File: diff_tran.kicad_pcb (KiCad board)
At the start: 2 copper layers, 28.7 x 13.8 mm, 30 parts, among them IC1 SN65LVDM176, IC2 SN65LVDM176, IC3 SN65LVDM176, IC4 SN65LVDM176, J1 SOLDER_JUMPER, J10 SOLDER_JUMPER, J11 SOLDER_JUMPER, J12 SOLDER_JUMPER, J2 SOLDER_JUMPER, J3 SOLDER_JUMPER, J4 SOLDER_JUMPER, J5 SOLDER_JUMPER, J6 SOLDER_JUMPER, J7 SOLDER_JUMPER, J8 SOLDER_JUMPER, J9 SOLDER_JUMPER, P1 CONN_02X03, P2 CONN_02X05

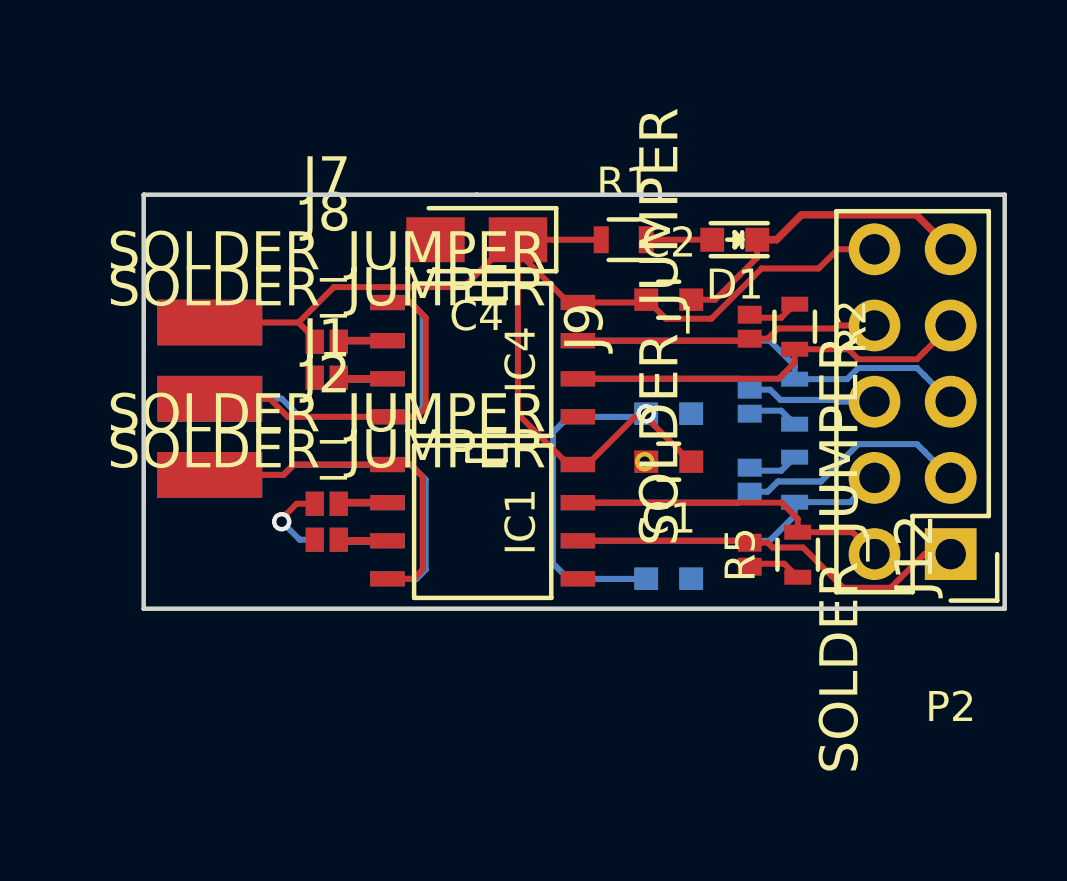
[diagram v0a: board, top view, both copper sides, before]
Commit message: Added some text, almost finished
Added some text, almost finished
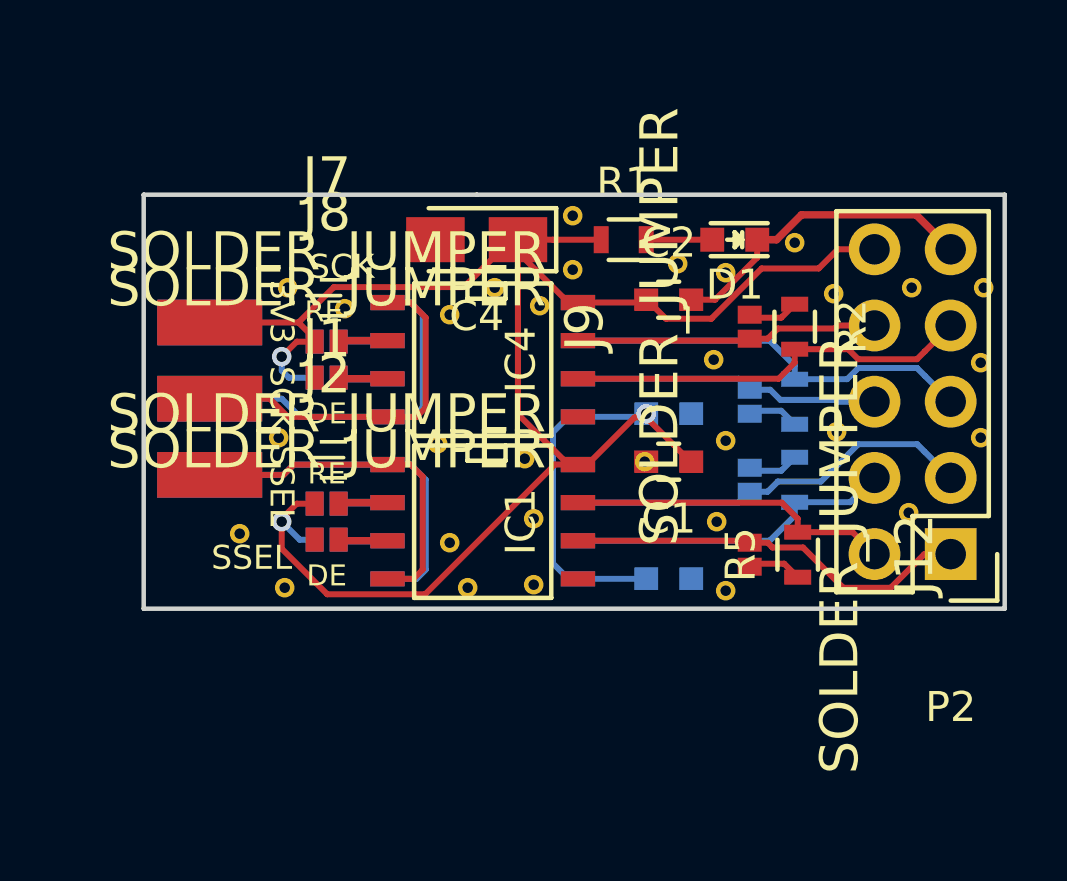
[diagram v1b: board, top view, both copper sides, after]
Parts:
- added ?: , LercheTech:Lerche_via_0.35_GND_MaskOver, F.Cu at (142.5, 103.0)
- added ?: , LercheTech:Lerche_via_0.35_GND_MaskOver, F.Cu at (155.0, 100.6)
- added ?: , LercheTech:Lerche_via_0.35_GND_MaskOver, F.Cu at (148.9, 103.2)
- added ?: , LercheTech:Lerche_via_0.35_GND_MaskOver, F.Cu at (148.6, 100.9)
- added ?: , LercheTech:Lerche_via_0.35_GND_MaskOver, F.Cu at (148.9, 98.2)
- added ?: , LercheTech:Lerche_via_0.35_GND_MaskOver, F.Cu at (148.5, 95.5)
- added ?: , LercheTech:Lerche_via_0.35_GND_MaskOver, F.Cu at (147.3, 92.3)
- added ?: , LercheTech:Lerche_via_0.35_GND_MaskOver, F.Cu at (143.8, 90.7)
- added ?: , LercheTech:Lerche_via_0.35_GND_MaskOver, F.Cu at (143.8, 92.5)
- added ?: , LercheTech:Lerche_via_0.35_GND_MaskOver, F.Cu at (142.7, 93.7)
- added ?: , LercheTech:Lerche_via_0.35_GND_MaskOver, F.Cu at (141.2, 93.1)
- added ?: , LercheTech:Lerche_via_0.35_GND_MaskOver, F.Cu at (152.6, 97.9)
- added ?: , LercheTech:Lerche_via_0.35_GND_MaskOver, F.Cu at (142.2, 98.8)
- added ?: , LercheTech:Lerche_via_0.35_GND_MaskOver, F.Cu at (142.5, 100.8)
- added ?: , LercheTech:Lerche_via_0.35_GND_MaskOver, F.Cu at (136.2, 93.8)
- added ?: , LercheTech:Lerche_via_0.35_GND_MaskOver, F.Cu at (132.7, 101.3)
- added ?: , LercheTech:Lerche_via_0.35_GND_MaskOver, F.Cu at (134.2, 103.1)
- added ?: , LercheTech:Lerche_via_0.35_GND_MaskOver, F.Cu at (140.3, 103.1)
- added ?: , LercheTech:Lerche_via_0.35_GND_MaskOver, F.Cu at (139.7, 101.6)
- added ?: , LercheTech:Lerche_via_0.35_GND_MaskOver, F.Cu at (139.3, 98.3)
- added ?: , LercheTech:Lerche_via_0.35_GND_MaskOver, F.Cu at (134.0, 98.1)
- added ?: , LercheTech:Lerche_via_0.35_GND_MaskOver, F.Cu at (139.7, 94.0)
- added ?: , LercheTech:Lerche_via_0.35_GND_MaskOver, F.Cu at (152.5, 93.3)
- added ?: , LercheTech:Lerche_via_0.35_GND_MaskOver, F.Cu at (134.3, 93.1)
- added ?: , LercheTech:Lerche_via_0.35_GND_MaskOver, F.Cu at (148.9, 92.6)
- added ?: , LercheTech:Lerche_via_0.35_GND_MaskOver, F.Cu at (151.2, 91.6)
- added ?: , LercheTech:Lerche_via_0.35_GND_MaskOver, F.Cu at (157.5, 93.1)
- added ?: , LercheTech:Lerche_via_0.35_GND_MaskOver, F.Cu at (155.1, 93.1)
- added ?: , LercheTech:Lerche_via_0.35_GND_MaskOver, F.Cu at (157.4, 95.6)
- added ?: , LercheTech:Lerche_via_0.35_GND_MaskOver, F.Cu at (157.4, 98.1)
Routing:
- net +3V3: track 56.7 -> 72.8 mm, vias 2 -> 3
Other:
- board text added: "3V3"
- board text added: "DE"
- board text added: "GND"
- board text added: "MISO"
- board text added: "MOSI"
- board text added: "SCK"
- board text added: "SSEL"
- board text added: "~RE"
